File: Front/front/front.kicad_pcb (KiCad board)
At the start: 2 copper layers, 28.5 x 51.8 mm, 14 parts, among them J1 Conn_01x10_Male, J2 JST 1mm Connector, SW1 SW_Push, U1 L293D

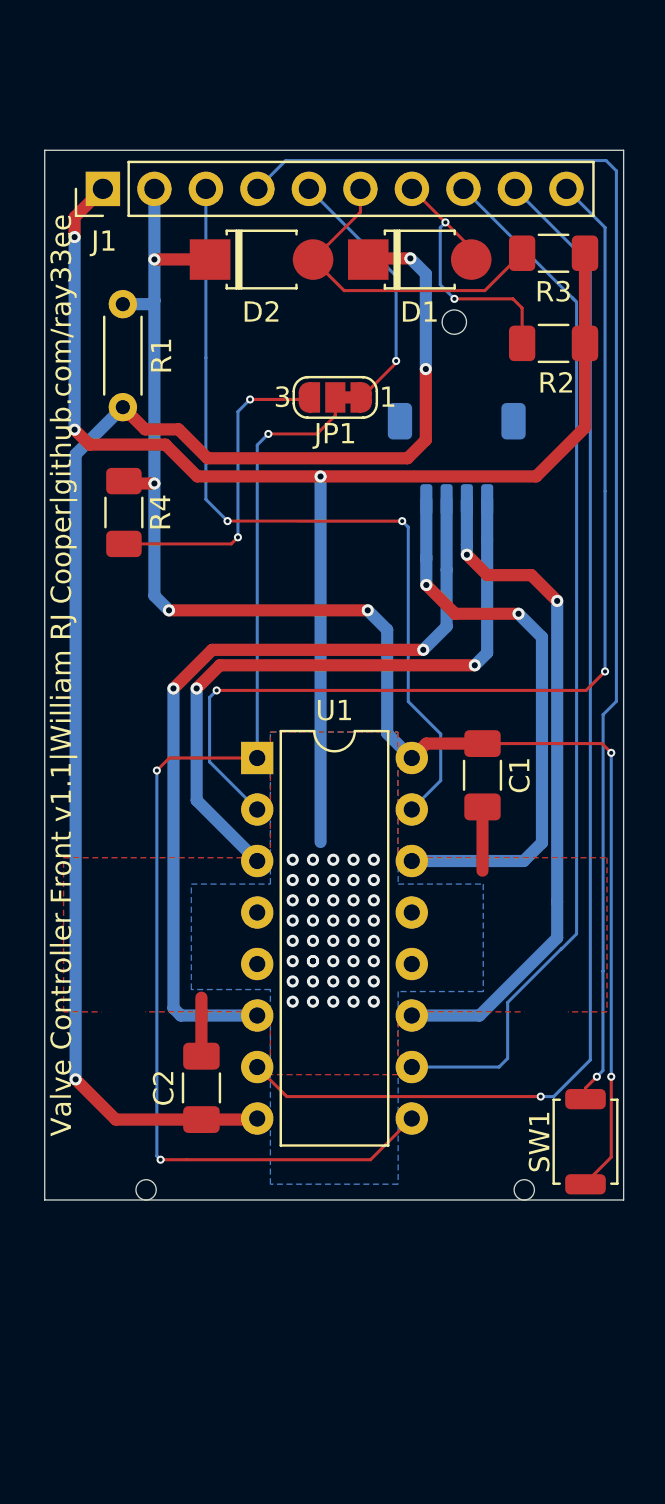
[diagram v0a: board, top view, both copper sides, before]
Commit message: Version 0.1.15 - Various changes, see changelog
Signed-off-by: ray33ee <30669752+ray33ee@users.noreply.github.com>
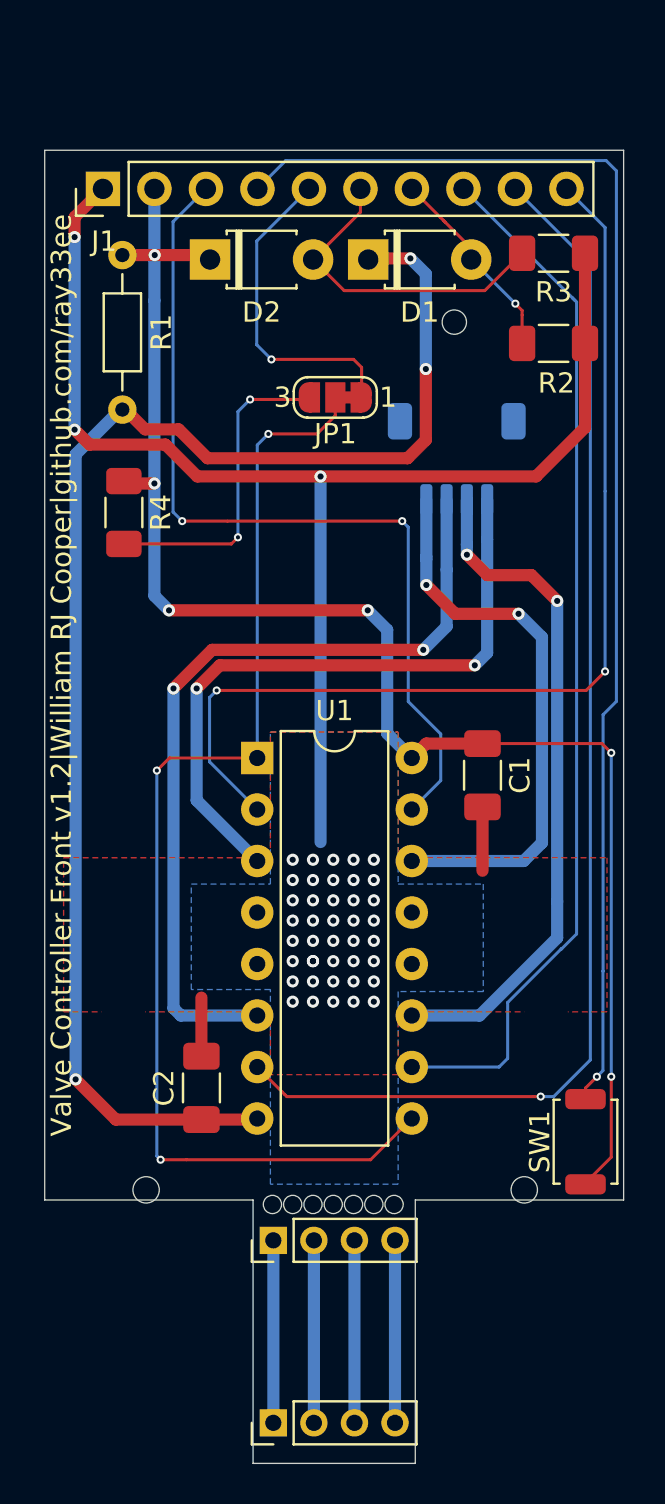
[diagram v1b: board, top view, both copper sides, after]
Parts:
- added REF**: MountingHole_2.1mm, MountingHole:MountingHole_2.1mm, F.Cu at (209.0, 132.0)
- added REF**: MountingHole_2.1mm, MountingHole:MountingHole_2.1mm, F.Cu at (208.0, 132.0)
- added REF**: MountingHole_2.1mm, MountingHole:MountingHole_2.1mm, F.Cu at (207.0, 132.0)
- added REF**: MountingHole_2.1mm, MountingHole:MountingHole_2.1mm, F.Cu at (206.0, 132.0)
- added REF**: MountingHole_2.1mm, MountingHole:MountingHole_2.1mm, F.Cu at (205.0, 132.0)
- added REF**: MountingHole_2.1mm, MountingHole:MountingHole_2.1mm, F.Cu at (204.0, 132.0)
- added REF**: MountingHole_2.1mm, MountingHole:MountingHole_2.1mm, F.Cu at (203.0, 132.0)
- added REF**: PinHeader_1x04_P2.00mm_Vertical, Connector_PinHeader_2.00mm:PinHeader_1x04_P2.00mm_Vertical, F.Cu at (203.0, 142.8)
- added REF**: PinHeader_1x04_P2.00mm_Vertical, Connector_PinHeader_2.00mm:PinHeader_1x04_P2.00mm_Vertical, F.Cu at (203.0, 133.8)
- R1: footprint Resistor_THT:R_Axial_DIN0204_L3.6mm_D1.6mm_P5.08mm_Horizontal -> Resistor_THT:R_Axial_DIN0204_L3.6mm_D1.6mm_P7.62mm_Horizontal
- moved R1 2.42 mm to (195.6, 85.2)
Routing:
- net (no net): track 0.00 -> 36.0 mm
- net /Diff_P2: track 16.3 -> 12.1 mm, vias 2 -> 1
- net /Enable_Controlled: track 12.8 -> 15.9 mm
- net /Coil_B2: track 41.0 -> 43.7 mm
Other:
- board size 28.5 x 51.8 mm -> 28.5 x 64.8 mm
- board text added: "Valve Controller Front v1.2|William RJ Cooper|github.com/ray33ee"
- board text removed: "Valve Controller Front v1.1|William RJ Cooper|github.com/ray33ee"

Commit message: Version 0.1.16 - Various changes, see changelog
Signed-off-by: ray33ee <30669752+ray33ee@users.noreply.github.com>
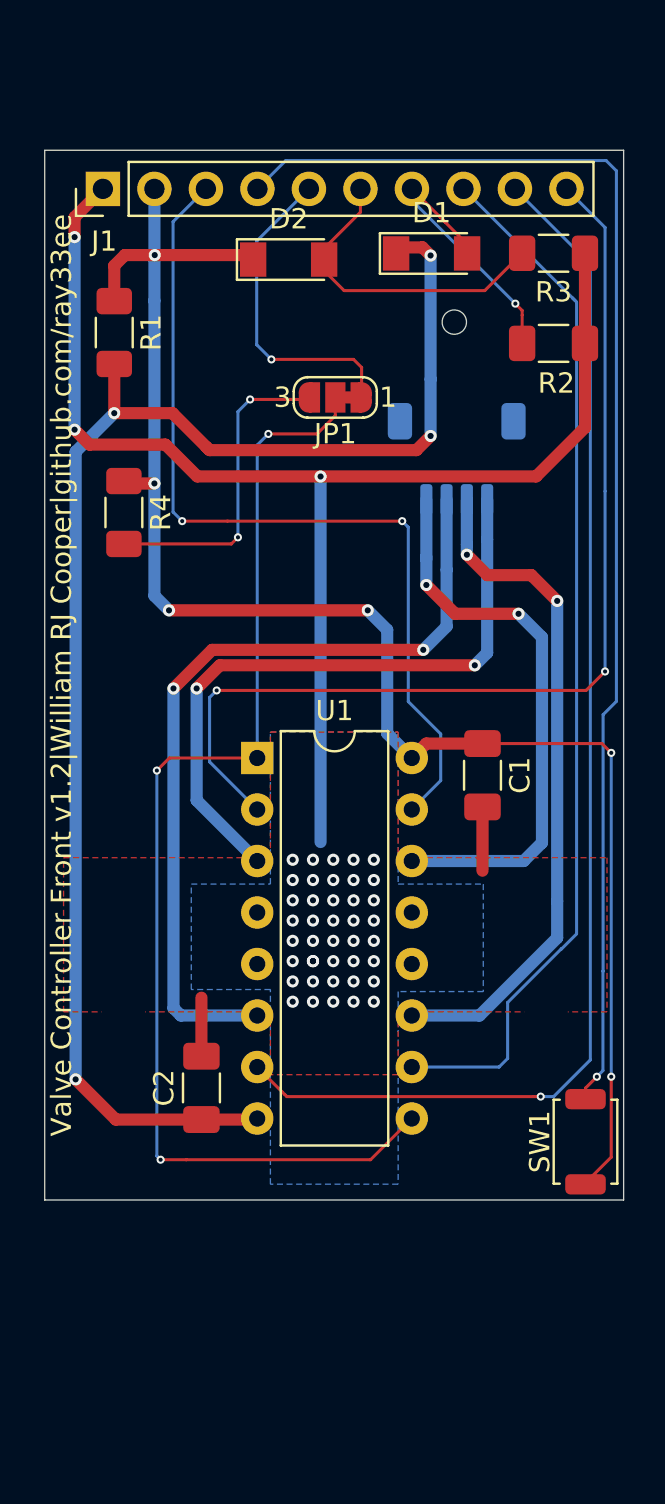
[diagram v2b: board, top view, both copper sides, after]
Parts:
- removed the REF** at (209.0, 132.0)
- removed the REF** at (208.0, 132.0)
- removed the REF** at (207.0, 132.0)
- removed the REF** at (206.0, 132.0)
- removed the REF** at (205.0, 132.0)
- removed the REF** at (204.0, 132.0)
- removed the REF** at (203.0, 132.0)
- removed the REF** at (203.0, 142.8)
- removed the REF** at (203.0, 133.8)
- D1, D2: footprint Diode_SMD:D_T-1_P5.08mm_Horizontal_SurfaceMount -> Diode_SMD:D_MiniMELF
- R1: footprint Resistor_THT:R_Axial_DIN0204_L3.6mm_D1.6mm_P7.62mm_Horizontal -> Resistor_SMD:R_1206_3216Metric_Pad1.30x1.75mm_HandSolder
- moved D2 3.88 mm to (203.8, 85.4)
- moved R1 3.84 mm to (195.2, 89.0)
- moved D1 3.14 mm to (210.8, 85.1)
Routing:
- net (no net): track 36.0 -> 0.00 mm
- net +5V: track 77.2 -> 81.7 mm
- net /Diff_P2: track 12.1 -> 16.3 mm
- net /Motor_Supply_Pre: track 71.6 -> 73.4 mm, vias 3 -> 4
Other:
- board size 28.5 x 64.8 mm -> 28.5 x 51.8 mm
